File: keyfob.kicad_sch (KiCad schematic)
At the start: 17 parts, among them J2 USB_A, SW2 SW_SPDT_321, U1 ATtiny85V-10S

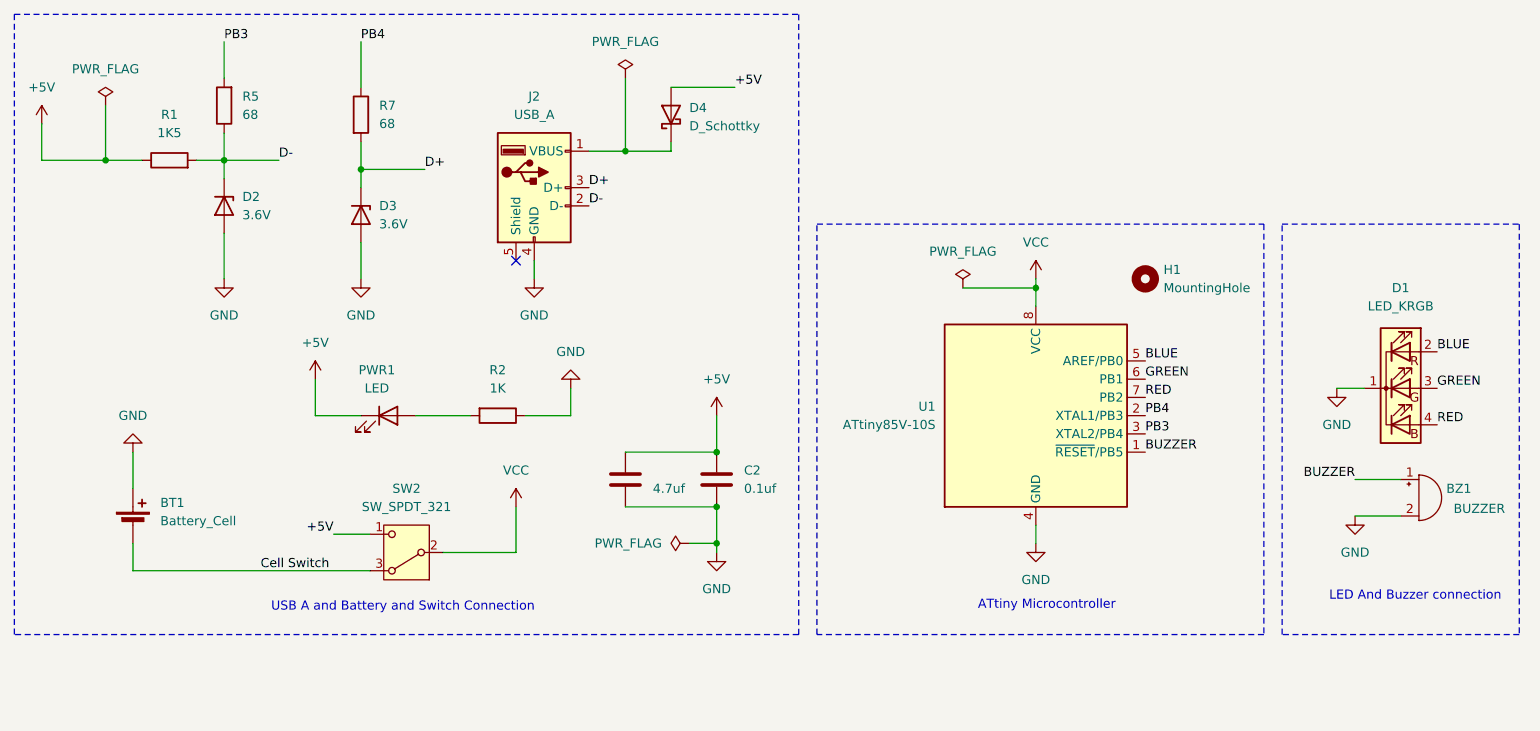
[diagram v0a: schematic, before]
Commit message: Upadated the Schematic and PCB Design
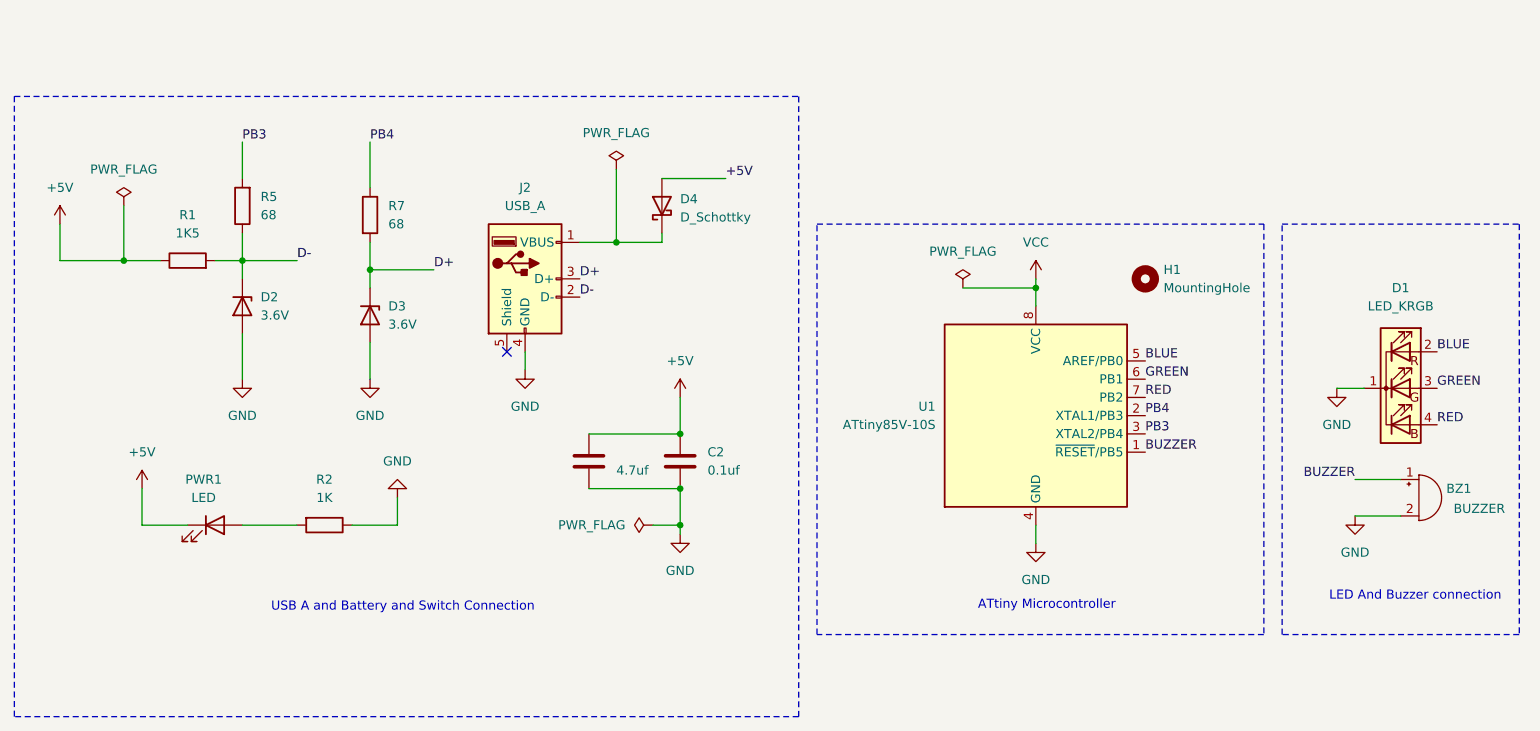
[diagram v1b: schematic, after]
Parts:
- removed BT1: Battery_Cell, symbol Device:Battery_Cell
- removed SW2: SW_SPDT_321, symbol Switch:SW_SPDT_321
- BZ1: footprint (none) -> Buzzer_Beeper:Buzzer_15x7.5RM7.6
- C1, C2: footprint (none) -> Capacitor_SMD:C_Elec_3x5.4
- D1: footprint (none) -> LED_SMD:LED_RGB_1210
- D2, D3, D4: footprint (none) -> Diode_SMD:D_0805_2012Metric
- H1: footprint (none) -> MountingHole:MountingHole_4mm
- J2: footprint (none) -> Connector_USB:USB_A_Molex_67643_Horizontal
- PWR1: footprint (none) -> LED_SMD:LED_0805_2012Metric
- R1, R2, R5, R7: footprint (none) -> Resistor_SMD:R_0805_2012Metric
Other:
- moved on the sheet: C2, D2, D3, D4, J2, PWR1, R1, R2, R5, R7

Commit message: PCB layout done
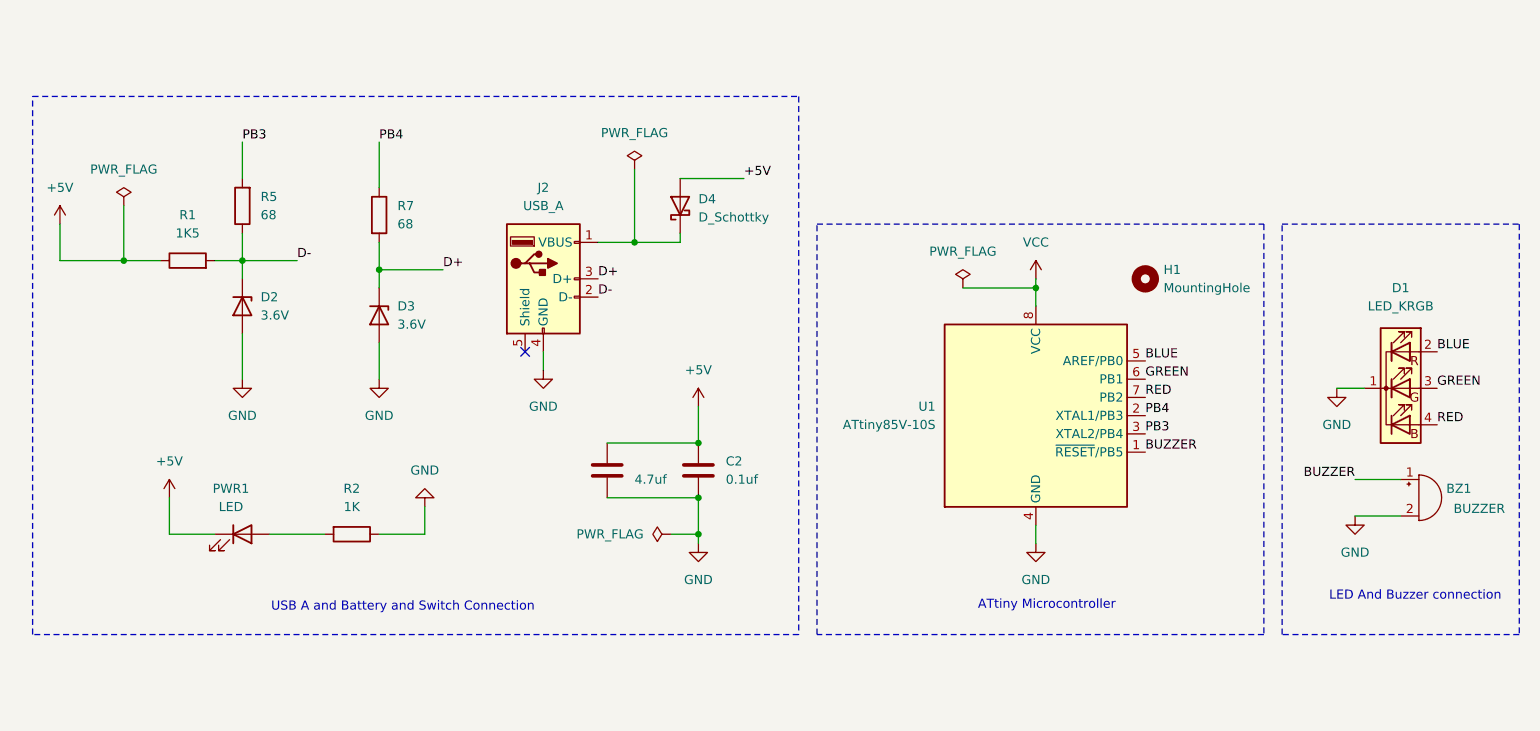
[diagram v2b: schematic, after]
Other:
- moved on the sheet: C2, D3, D4, J2, PWR1, R2, R7
